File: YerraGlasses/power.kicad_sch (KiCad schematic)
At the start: 8 parts, among them SW1 SW_SPDT, U4 RT9013-33GB

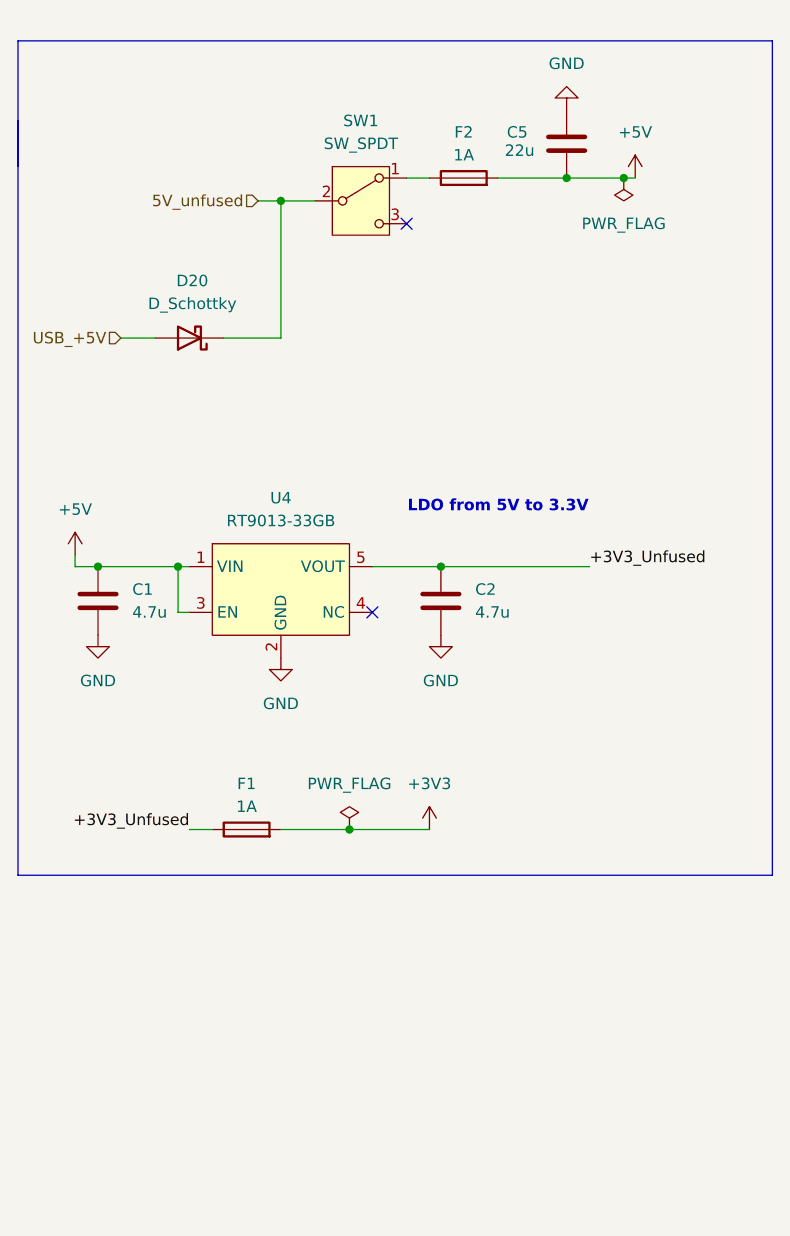
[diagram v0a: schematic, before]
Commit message: cad completion prototype
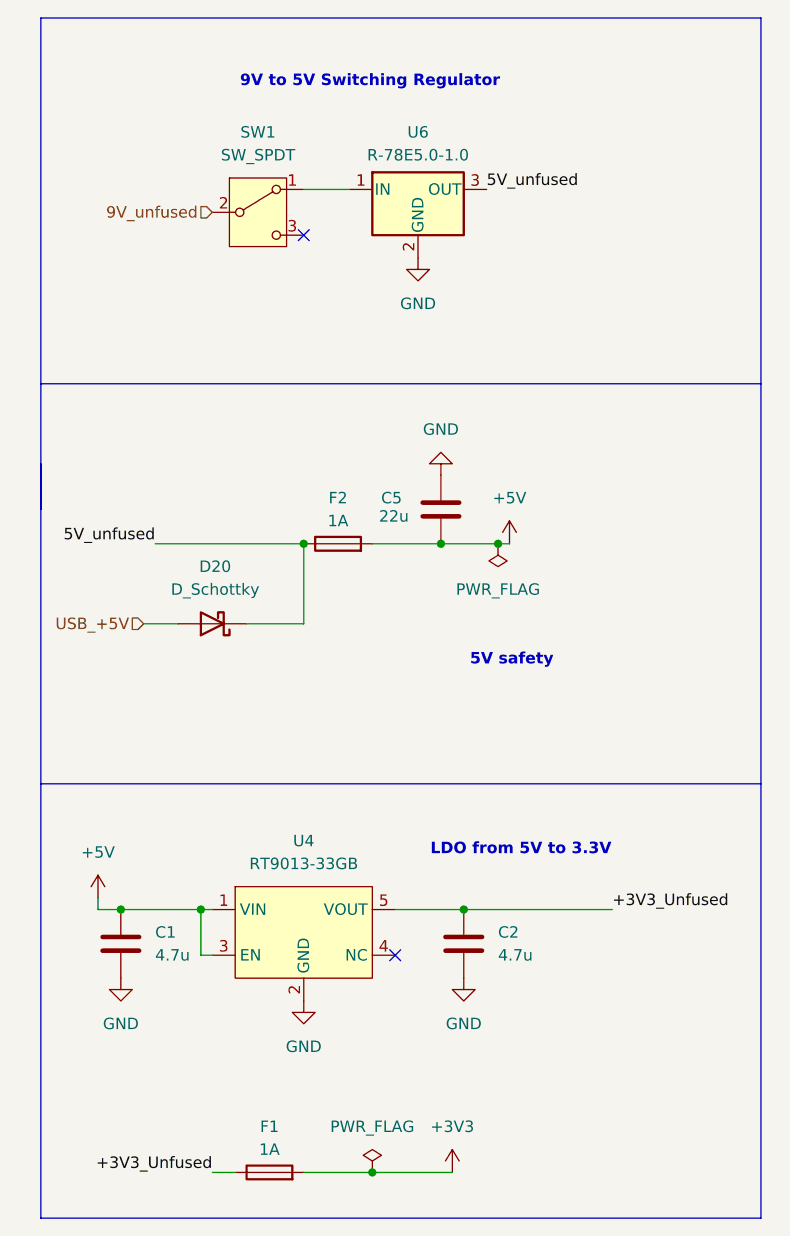
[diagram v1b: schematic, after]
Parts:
- added U6: R-78E5.0-1.0, Converter_DCDC:Converter_DCDC_RECOM_R-78E-0.5_THT, symbol Regulator_Switching:R-78E5.0-1.0
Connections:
- net 5V_unfused: now also F2.1, U6.3 (OUT); no longer SW1.2 (B)
- net GND: now also U6.2 (GND)
- net at SW1.1 (A): now also U6.1 (IN); no longer F2.1
- new net 9V_unfused: SW1.2 (B)
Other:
- note added: "5V safety"
- note added: "9V to 5V Switching Regulator"
- moved on the sheet: C1, C2, C5, D20, F1, F2, SW1, U4
